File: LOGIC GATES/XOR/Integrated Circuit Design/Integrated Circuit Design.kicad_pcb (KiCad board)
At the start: 2 copper layers, 25 x 40 mm, 0 parts

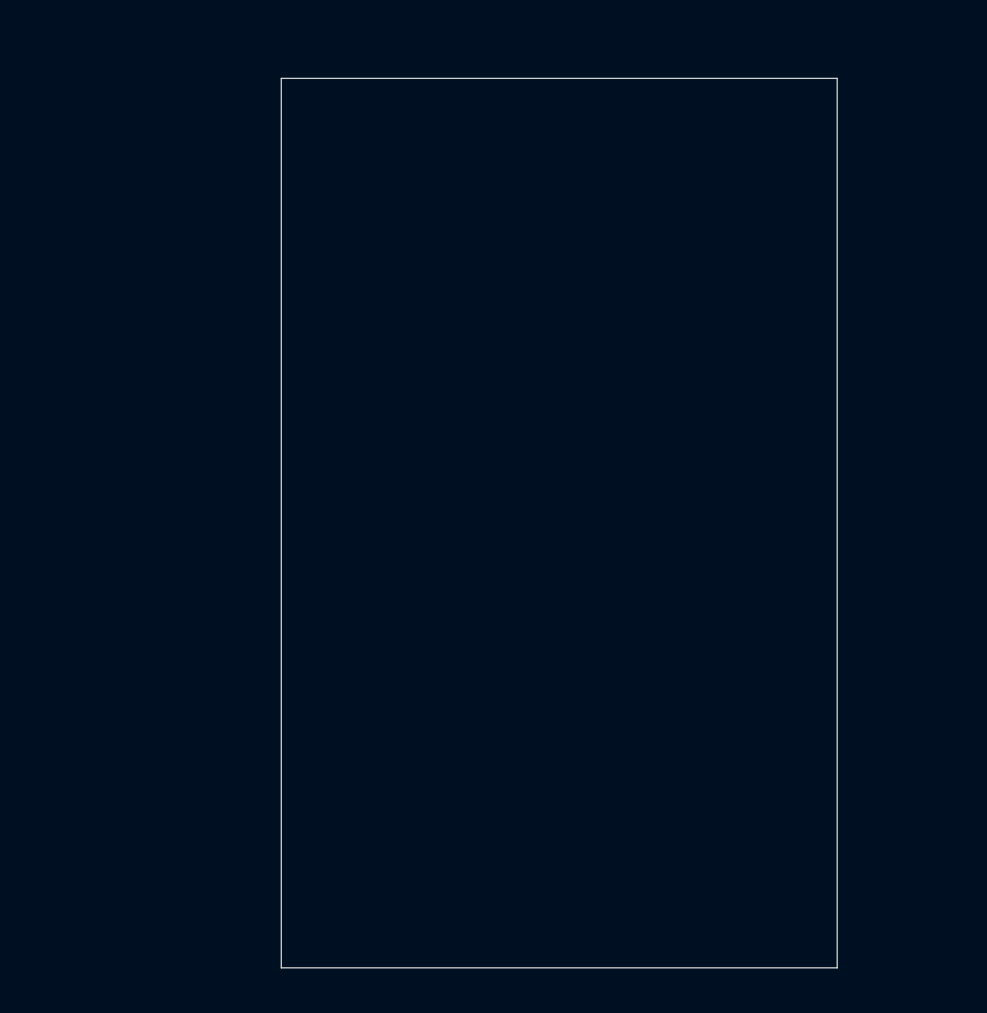
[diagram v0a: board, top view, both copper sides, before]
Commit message: Auto-update: 22.12.2025 16:16:21,18
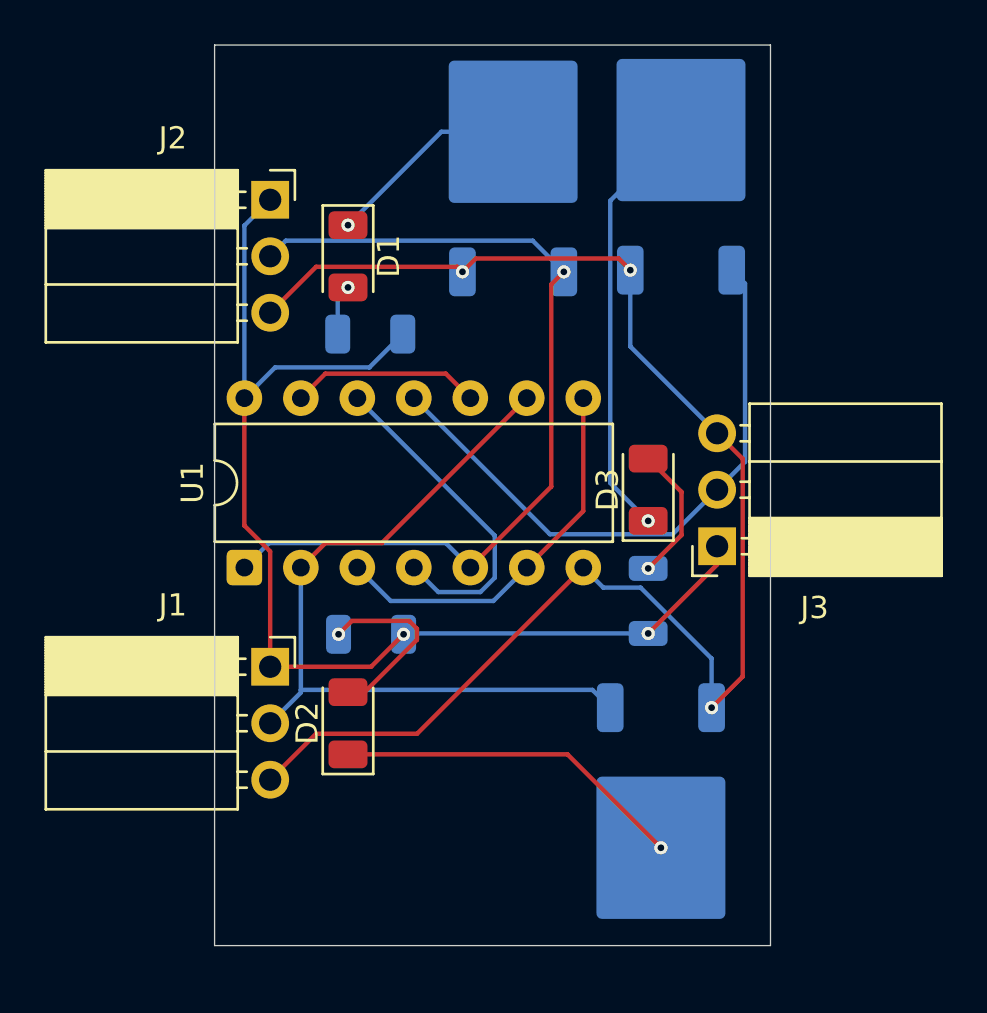
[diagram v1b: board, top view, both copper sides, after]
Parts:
- added D1: LED, LED_SMD:LED_1206_3216Metric, F.Cu at (111.0, 84.5)
- added D2: LED, LED_SMD:LED_1206_3216Metric, F.Cu at (111.0, 105.5)
- added D3: LED, LED_SMD:LED_1206_3216Metric, F.Cu at (124.5, 95.0)
- added J1: Conn_01x03_Socket, Connector_PinSocket_2.54mm:PinSocket_1x03_P2.54mm_Horizontal, F.Cu at (107.5, 103.0)
- added J2: Conn_01x03_Socket, Connector_PinSocket_2.54mm:PinSocket_1x03_P2.54mm_Horizontal, F.Cu at (107.5, 82.0)
- added J3: Conn_01x03_Socket, Connector_PinSocket_2.54mm:PinSocket_1x03_P2.54mm_Horizontal, F.Cu at (127.6, 97.5)
- added Q1: QM6006D, Package_TO_SOT_SMD:TO-252-2, B.Cu at (118.4, 80.2)
- added Q2: QM6006D, Package_TO_SOT_SMD:TO-252-2, B.Cu at (125.1, 109.8)
- added Q3: QM6006D, Package_TO_SOT_SMD:TO-252-2, B.Cu at (126.0, 80.1)
- added R1: R, Resistor_SMD:R_1206_3216Metric, B.Cu at (112.0, 88.0)
- added R2: R, Resistor_SMD:R_1206_3216Metric, B.Cu at (112.0, 101.5)
- added R3: R, Resistor_SMD:R_1206_3216Metric, B.Cu at (124.5, 100.0)
- added U1: 4011, Package_DIP:DIP-14_W7.62mm, F.Cu at (106.3, 98.5)
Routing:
- net Net-(J1-Pin_3): track 0.00 -> 67.7 mm, vias 0 -> 3
- net Net-(J1-Pin_1): track 0.00 -> 53.1 mm, vias 0 -> 2
- net Net-(J2-Pin_2): track 0.00 -> 40.2 mm, vias 0 -> 1
- net Net-(J1-Pin_2): track 0.00 -> 35.1 mm
- net Net-(J3-Pin_2): track 0.00 -> 27.6 mm
- net Net-(D3-K): track 0.00 -> 19.6 mm, vias 0 -> 1
- net Net-(U1-Pad3): track 0.00 -> 17.5 mm
- net Net-(D2-K): track 0.00 -> 15.8 mm, vias 0 -> 1
- net Net-(U1-Pad12): track 0.00 -> 15.0 mm
- net Net-(D1-K): track 0.00 -> 9.17 mm, vias 0 -> 1
- net Net-(U1-Pad10): track 0.00 -> 8.53 mm
- net Net-(D2-A): track 0.00 -> 8.49 mm, vias 0 -> 1
- net Net-(D3-A): track 0.00 -> 6.18 mm, vias 0 -> 1
- net Net-(D1-A): track 0.00 -> 2.29 mm, vias 0 -> 1
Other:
- board size 25 x 40 mm -> 25 x 40.5 mm
